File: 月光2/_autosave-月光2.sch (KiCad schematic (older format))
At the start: 69 parts, among them J1 Conn_01x12, J2 Conn_01x12, J3 Conn_01x05, J4 Conn_01x03, J6 Conn_01x02, Q5 IRLML6344TRPBFTR, SW1 SW_Push_Dual_x2, U1 DRV8835, U2 STM32F413CH6, U3 LED_FOTR, U4 LP5907_DBV, U5 ICM20648, U6 LED_FOTR, U7 LED_FOTR, U8 LED_FOTR, Y1 Crystal_GND23

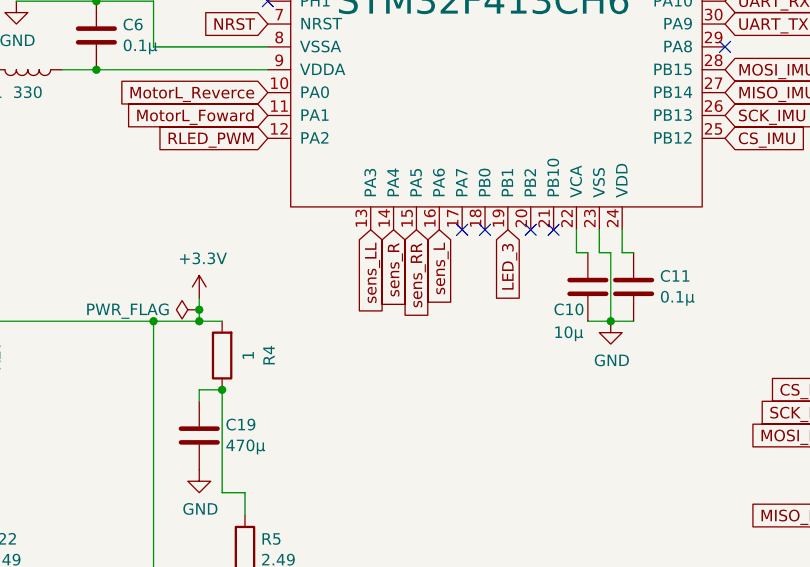
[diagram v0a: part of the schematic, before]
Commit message: finish 3
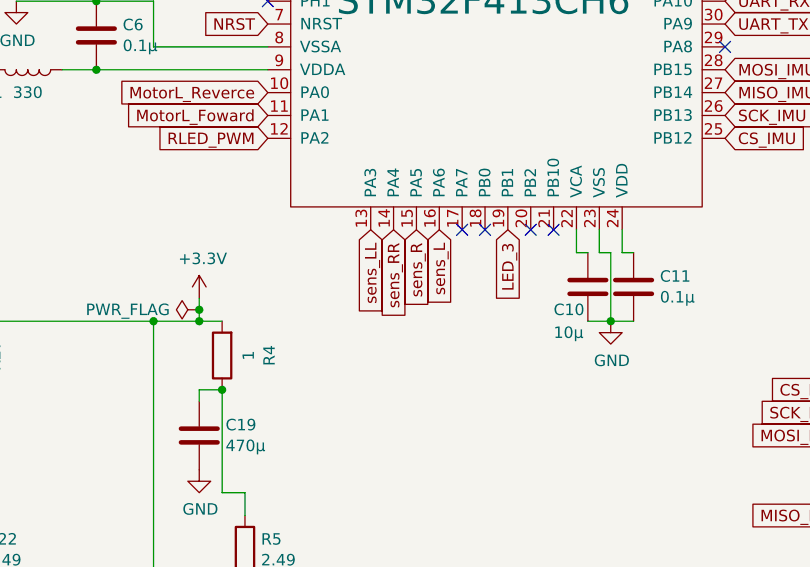
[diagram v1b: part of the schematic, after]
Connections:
- net sens_R: now also U2.15 (PA5); no longer U2.14 (PA4)
- net sens_RR: now also U2.14 (PA4); no longer U2.15 (PA5)
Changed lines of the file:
@@
 sens_L
 Text GLabel 5700 5100 3    50   Input ~ 0
+sens_R
+Text GLabel 5600 5100 3    50   Input ~ 0
 sens_RR
-Text GLabel 5600 5100 3    50   Input ~ 0
-sens_R
 Text GLabel 5500 5100 3    50   Input ~ 0
 sens_LL
